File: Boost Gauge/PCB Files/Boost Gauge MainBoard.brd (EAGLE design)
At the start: 88 x 63 mm, 76 parts, among them IC1 MCT6SD, IC2 MCP96RL00-E_MX, IC4 ATMEGA328PB-AN, IC6 7805DT, IC7 MCP25625-E_SS, Q1 BUK7Y6R0-60EX

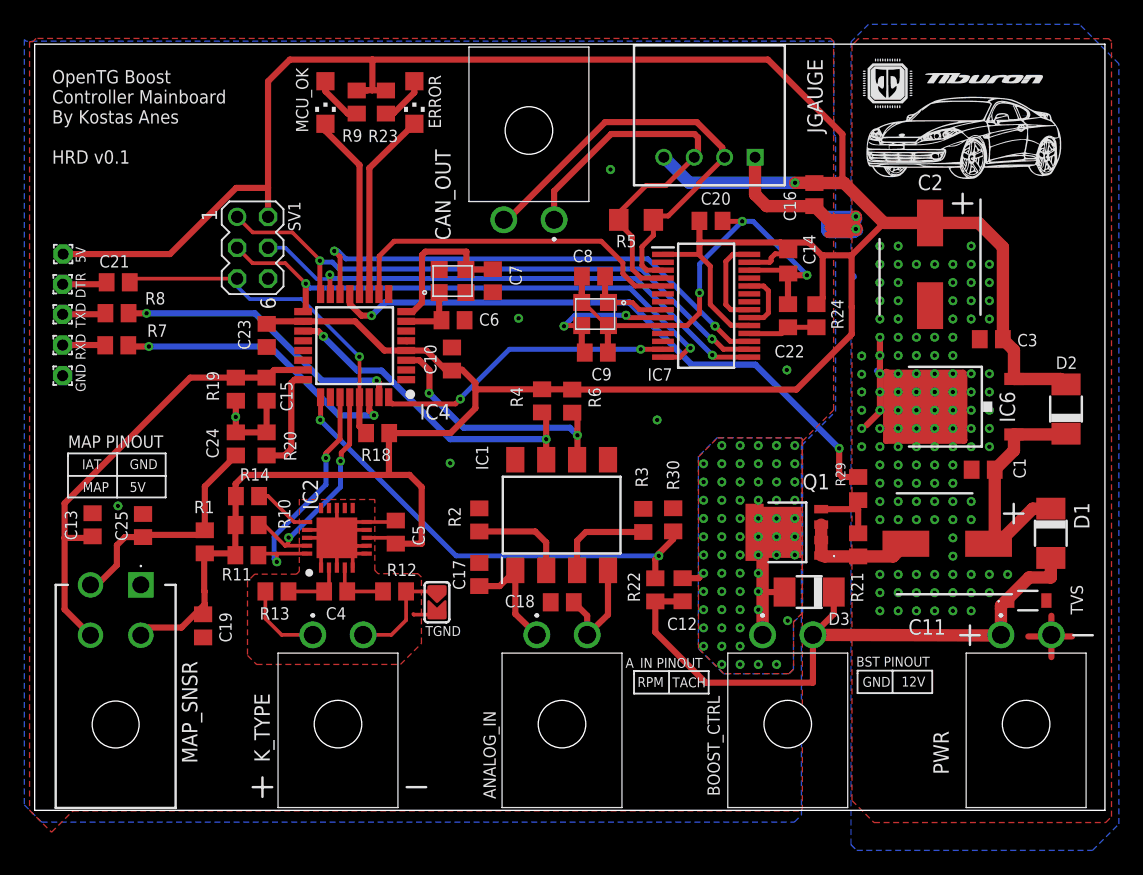
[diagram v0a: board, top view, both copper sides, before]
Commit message: v0.2 PCB
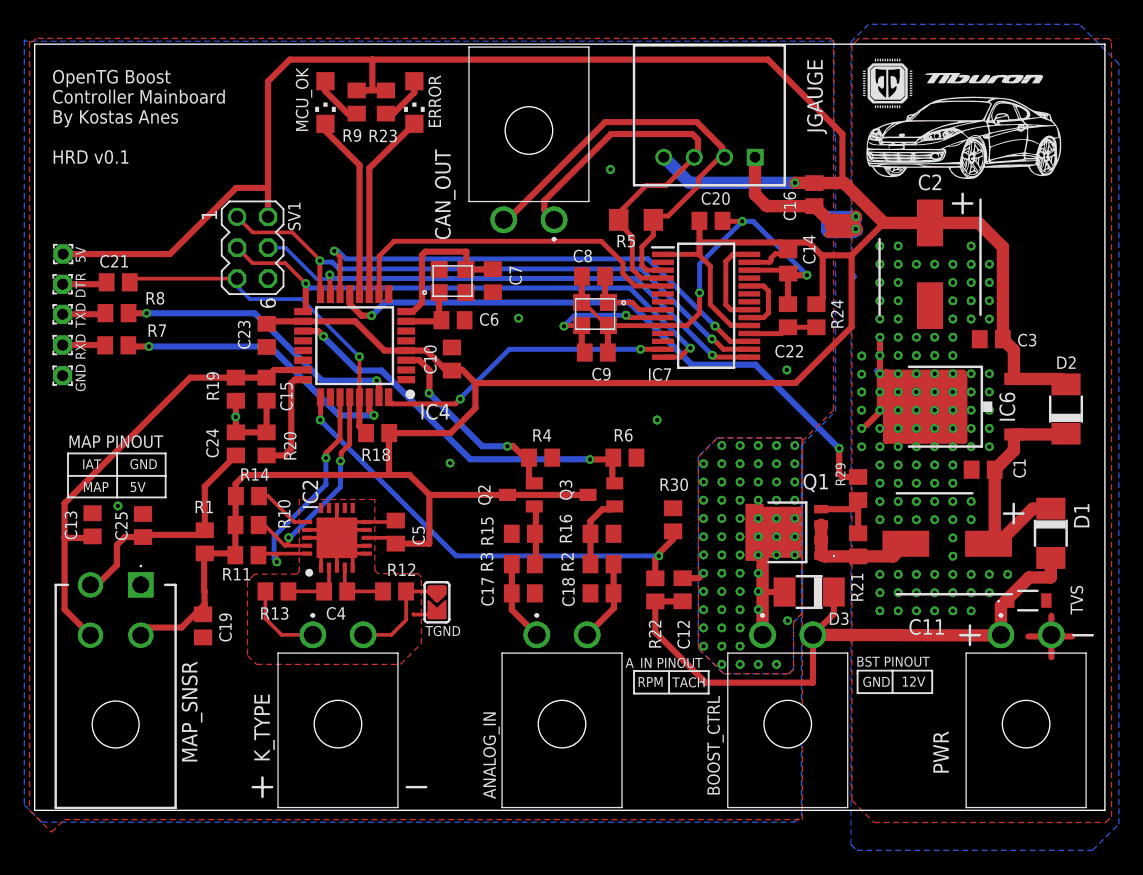
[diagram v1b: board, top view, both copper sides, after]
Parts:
- removed IC1: MCT6SD, MCT6SD:SOP254P1016X385-8N
- added Q2, Q3: BC817-40LT1SMD, transistor-npn:SOT23-BEC
- added R15, R16: 100k, rcl:R0805
- moved R2 10.7 mm to (46.6, 20.2), turned to 0 degrees
- moved R3 10.5 mm to (40.2, 20.2), turned to 180 degrees
- moved R6 6.35 mm to (48.5, 29.0), turned to 180 degrees
- moved R4 4.67 mm to (41.6, 29.0), turned to 180 degrees
- moved C17 3.94 mm to (40.2, 17.8), turned to 0 degrees
- moved C18 3.35 mm to (46.6, 17.8)
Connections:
- removed net N$2: IC1.2, R2.2
- new net N$4: Q3.B, R16.1, R2.1
- net +5V: now also Q2.C, Q3.C; no longer R4.2, R6.2
- net GND: now also R15.2, R16.2, R4.1, R6.1; no longer IC1.5, IC1.8, R2.1, R3.1
- net N$3: now also Q2.B, R15.1, R3.1; no longer IC1.3, R3.2
- net RPM_ISO: now also Q2.E, R4.2; no longer IC1.6, R6.1
- net RPM_SIGNAL: now also R3.2; no longer IC1.1
- net TACH_ISO: now also Q3.E, R6.2; no longer IC1.7, R4.1
- net TACH_SIGNAL: now also R2.2; no longer IC1.4
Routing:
- net +5V: track 296.0 -> 309.3 mm
- net N$4: track 0.00 -> 8.52 mm
- net N$2: track 8.17 -> 0.00 mm
- net RPM_ISO: track 22.0 -> 17.0 mm
- net TACH_ISO: track 28.0 -> 32.4 mm
- net RPM_SIGNAL: track 9.54 -> 6.66 mm
- net TACH_SIGNAL: track 9.16 -> 7.10 mm
- net N$3: track 8.18 -> 7.34 mm
- net CAN_H: track 34.0 -> 34.6 mm
